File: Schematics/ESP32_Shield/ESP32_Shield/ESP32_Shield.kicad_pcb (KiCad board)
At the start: 2 copper layers, 26.6 x 50.4 mm, 19 parts, among them J1 Conn_01x10, Q3 Si2319CDS, Q4 Si2319CDS, U6 ADS1234IPW, U7 SHT30-DIS

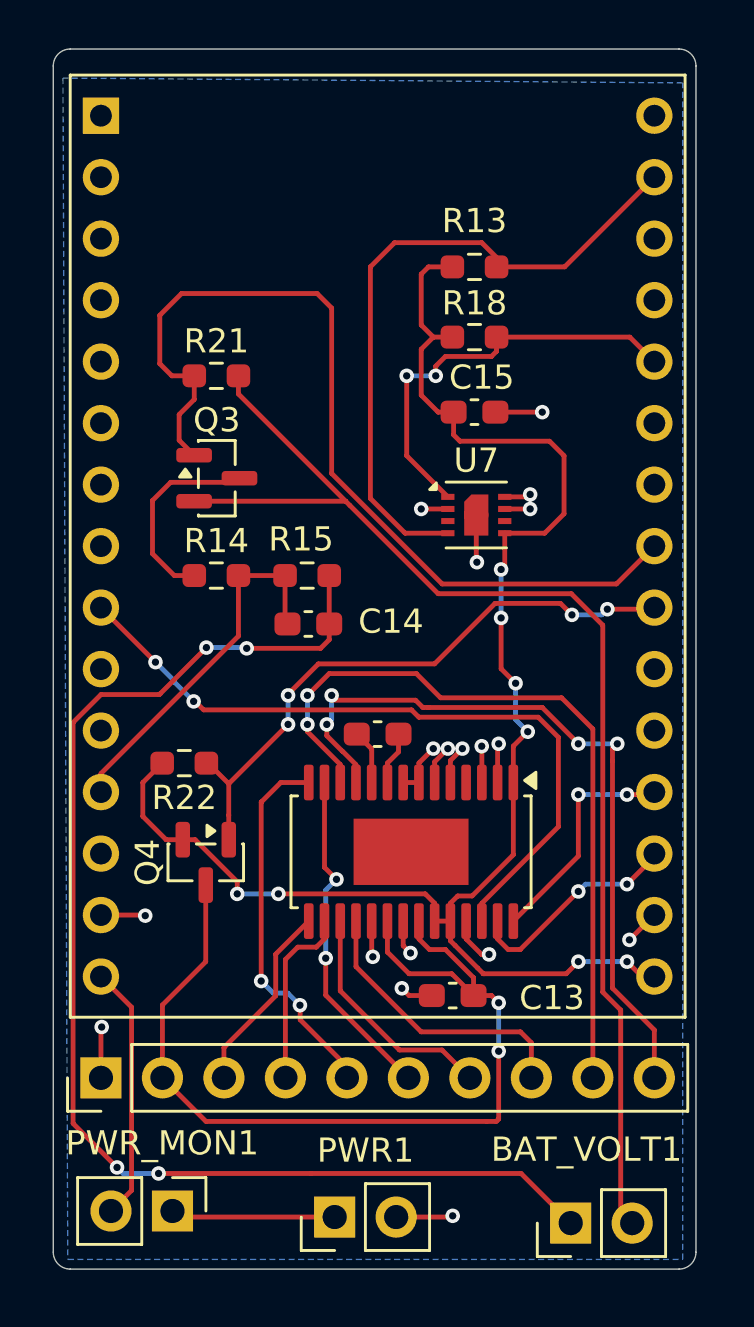
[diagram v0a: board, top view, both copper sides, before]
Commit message: korrekturen
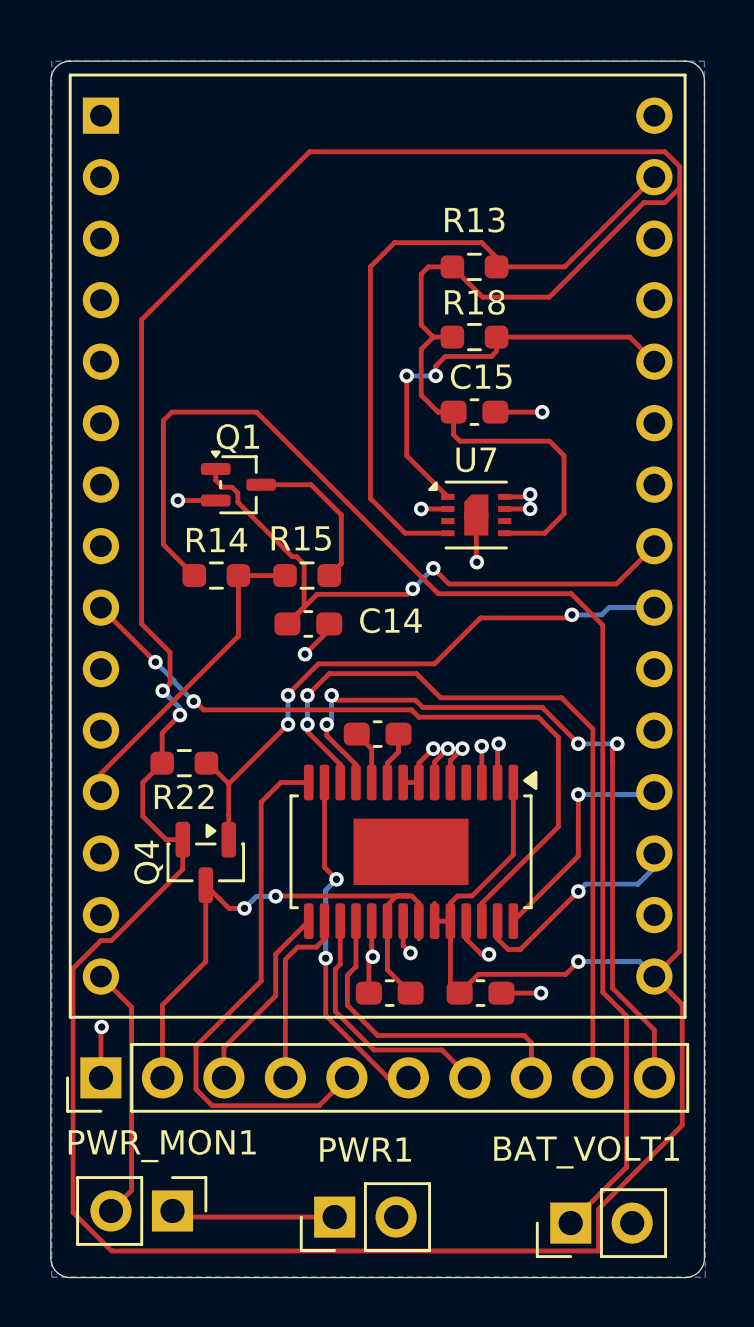
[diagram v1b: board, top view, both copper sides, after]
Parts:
- removed Q3: Si2319CDS, Package_TO_SOT_SMD:SOT-23
- removed R21: 100k, Resistor_SMD:R_0603_1608Metric_Pad0.98x0.95mm_HandSolder
- added C1: 0.1u, Capacitor_SMD:C_0603_1608Metric_Pad1.08x0.95mm_HandSolder, F.Cu at (128.2, 101.0)
- added Q1: Si1308EDL, Package_TO_SOT_SMD:SOT-323_SC-70, F.Cu at (118.2, 80.0)
- moved C13 2.60 mm to (124.5, 101.0)
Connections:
- BAT_VOLT1 pad 1: -BATT -> +BATT
- BAT_VOLT1 pad 2: +BATT -> GND
- C14 pad 1: -BATT -> GND
- C14 pad 2: bat_adc -> en_meas
- R14 pad 1: Net-(Q3-D) -> +BATT
- R15 pad 1: -BATT -> Net-(Q1-D)
- U2 pad 23: !en_meas -> en_meas
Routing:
- net +3.3V: track 66.6 -> 190.4 mm, vias 8 -> 3
- net -BATT: track 53.5 -> 0.00 mm, vias 4 -> 0
- net !en_meas: track 37.9 -> 0.00 mm
- net en_meas: track 0.00 -> 25.7 mm, vias 0 -> 2
- net Net-(J1-Pin_2): track 39.3 -> 24.8 mm
- net Net-(Q3-D): track 8.33 -> 0.00 mm
- net Net-(J1-Pin_5): track 15.5 -> 22.8 mm, vias 2 -> 0
- net Net-(Q1-D): track 0.00 -> 6.14 mm
- net +BATT: track 51.2 -> 54.9 mm
- net bat_adc: track 15.3 -> 13.2 mm
- net Net-(J1-Pin_8): track 11.9 -> 13.3 mm
- net Net-(J1-Pin_7): track 10.2 -> 11.0 mm
- net SCLK: track 9.11 -> 9.51 mm, vias 2 -> 1
- net !EN_DMS: track 25.3 -> 25.0 mm, vias 4 -> 3
- net D_RDY_OUT: track 9.52 -> 9.67 mm, vias 2 -> 1
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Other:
- board size 26.6 x 50.4 mm -> 27 x 50.2 mm
